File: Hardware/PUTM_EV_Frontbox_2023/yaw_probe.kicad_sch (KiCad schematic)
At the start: 10 parts, among them IC1 ELVH-MF12D-HRRJ-C-N3A4, IC2 ELVH-MF12D-HRRJ-C-N3A4

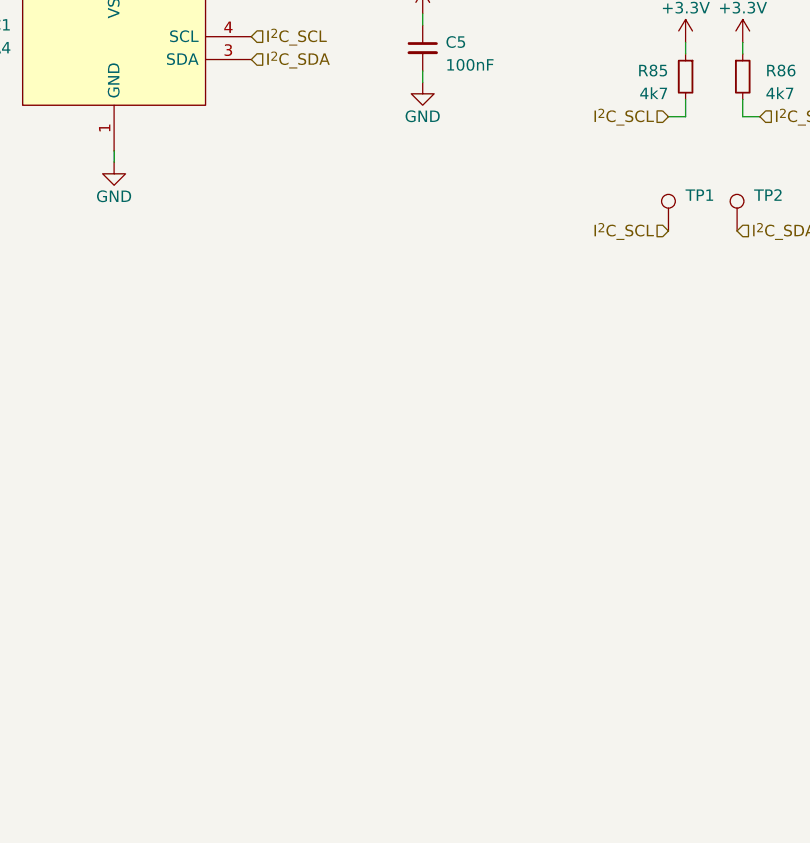
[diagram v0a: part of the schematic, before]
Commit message: Ready for production
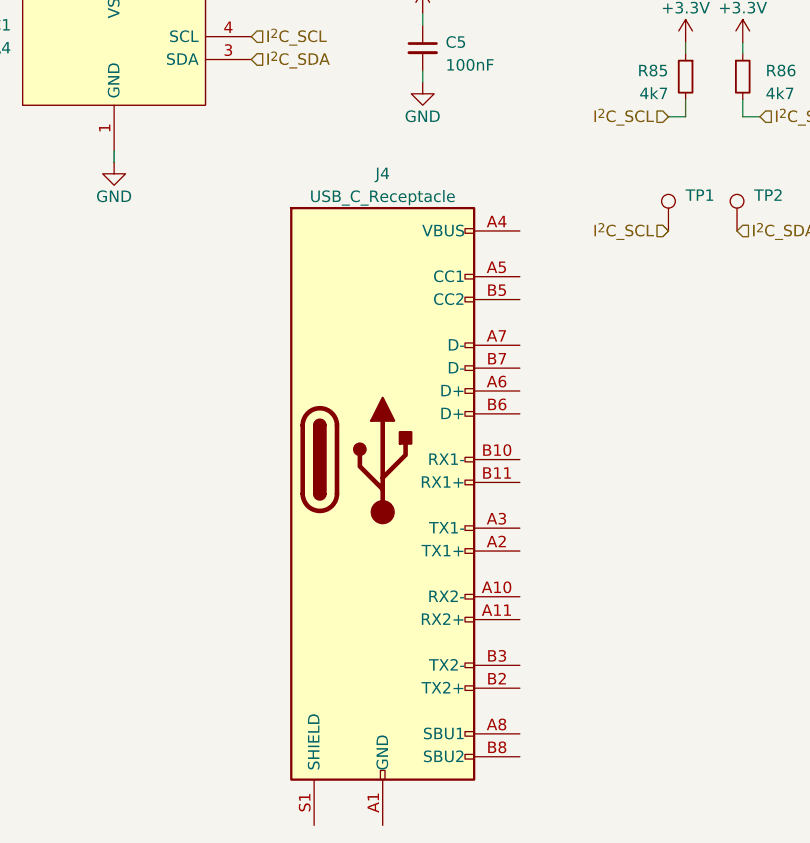
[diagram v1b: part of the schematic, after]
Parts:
- added J4: USB_C_Receptacle, Frontbox:CUI_UJ31-CH-31-SMT-TR, symbol Connector:USB_C_Receptacle
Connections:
- new net: J4.A1 (GND), J4.A12 (GND), J4.B1 (GND), J4.B12 (GND)
- new net: J4.A4 (VBUS), J4.A9 (VBUS), J4.B4 (VBUS), J4.B9 (VBUS)
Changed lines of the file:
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@@
+    )
+  )
+  (symbol (lib_id "Connector:USB_C_Receptacle") (at 105.41 141.605 0) (unit 1)
+    (in_bom yes) (on_board yes) (dnp no) (fields_autoplaced)
+    (property "Reference" "J4" (at 105.41 109.855 0)
+      (effects (font (size 1.27 1.27)))
+    )
+    (property "Value" "USB_C_Receptacle" (at 105.41 112.395 0)
+      (effects (font (size 1.27 1.27)))
+    )
+    (property "Footprint" "Frontbox:CUI_UJ31-CH-31-SMT-TR" (at 109.22 141.605 0)
+      (effects (font (size 1.27 1.27)) hide)
+    )
+    (property "Datasheet" "https://eu.mouser.com/ProductDetail/GCT/USB4085-GF-A?qs=KUoIvG%2F9Ilba1bQOahfWjw%3D%3D" (at 109.22 141.605 0)
+      (effects (font (size 1.27 1.27)) hide)
+    )
+    (pin "A1")
+    (pin "A10")
+    (pin "A11")
+    (pin "A12")
+    (pin "A2")
+    (pin "A3")
+    (pin "A4")
+    (pin "A5")
+    (pin "A6")
+    (pin "A7")
+    (pin "A8")
+    (pin "A9")
+    (pin "B1")
+    (pin "B10")
+    (pin "B11")
+    (pin "B12")
+    (pin "B2")
+    (pin "B3")
+    (pin "B4")
+    (pin "B5")
+    (pin "B6")
+    (pin "B7")
+    (pin "B8")
+    (pin "B9")
+    (pin "S1")
+    (instances
+      (project "PUTM_EV_Frontbox_2023"
+        (path "/b652b05a-4e3d-4ad1-b032-18886abe7d45"
+          (reference "J4") (unit 1)
+        )
+        (path "/b652b05a-4e3d-4ad1-b032-18886abe7d45/ba538a3c-1084-4770-aed2-08b4305d2379"
+          (reference "J4") (unit 1)
+        )
+      )
     )
   )

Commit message: PCB taken apart
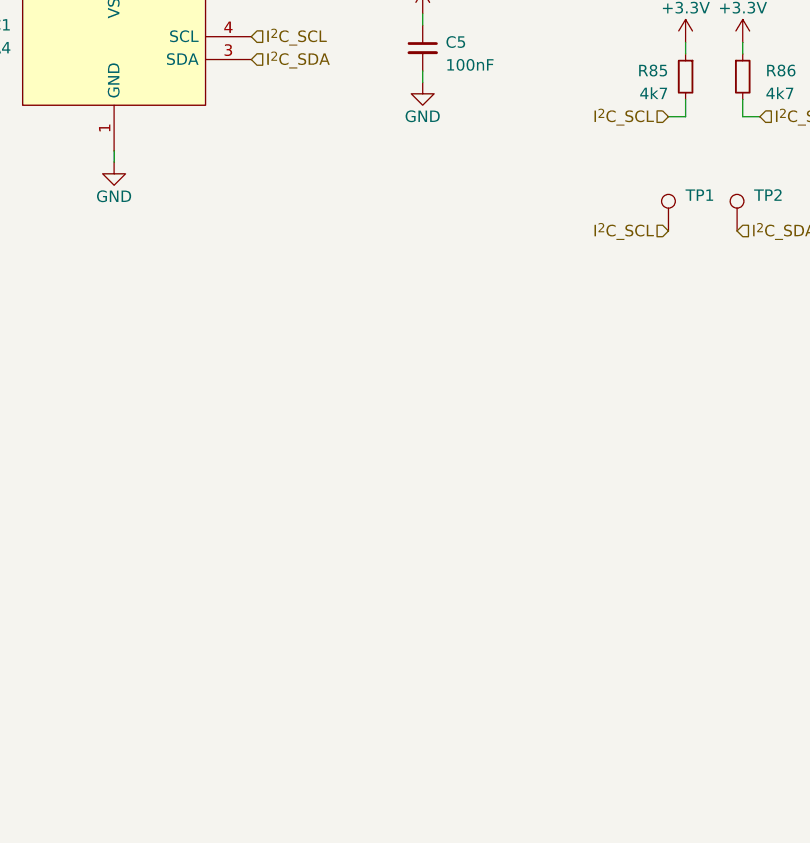
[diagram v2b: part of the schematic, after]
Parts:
- removed J4: USB_C_Receptacle, Frontbox:CUI_UJ31-CH-31-SMT-TR, symbol Connector:USB_C_Receptacle
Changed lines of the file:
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@@
-    )
-  )
-  (symbol (lib_id "Connector:USB_C_Receptacle") (at 105.41 141.605 0) (unit 1)
-    (in_bom yes) (on_board yes) (dnp no) (fields_autoplaced)
-    (property "Reference" "J4" (at 105.41 109.855 0)
-      (effects (font (size 1.27 1.27)))
-    )
-    (property "Value" "USB_C_Receptacle" (at 105.41 112.395 0)
-      (effects (font (size 1.27 1.27)))
-    )
-    (property "Footprint" "Frontbox:CUI_UJ31-CH-31-SMT-TR" (at 109.22 141.605 0)
-      (effects (font (size 1.27 1.27)) hide)
-    )
-    (property "Datasheet" "https://eu.mouser.com/ProductDetail/GCT/USB4085-GF-A?qs=KUoIvG%2F9Ilba1bQOahfWjw%3D%3D" (at 109.22 141.605 0)
-      (effects (font (size 1.27 1.27)) hide)
-    )
-    (pin "A1")
-    (pin "A10")
-    (pin "A11")
-    (pin "A12")
-    (pin "A2")
-    (pin "A3")
-    (pin "A4")
-    (pin "A5")
-    (pin "A6")
-    (pin "A7")
-    (pin "A8")
-    (pin "A9")
-    (pin "B1")
-    (pin "B10")
-    (pin "B11")
-    (pin "B12")
-    (pin "B2")
-    (pin "B3")
-    (pin "B4")
-    (pin "B5")
-    (pin "B6")
-    (pin "B7")
-    (pin "B8")
-    (pin "B9")
-    (pin "S1")
-    (instances
-      (project "PUTM_EV_Frontbox_2023"
-        (path "/b652b05a-4e3d-4ad1-b032-18886abe7d45"
-          (reference "J4") (unit 1)
-        )
-        (path "/b652b05a-4e3d-4ad1-b032-18886abe7d45/ba538a3c-1084-4770-aed2-08b4305d2379"
-          (reference "J4") (unit 1)
-        )
-      )
     )
   )
